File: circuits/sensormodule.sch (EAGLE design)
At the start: 9 parts, among them U1 ATMEGA328P_PDIP, Y1 16MHz

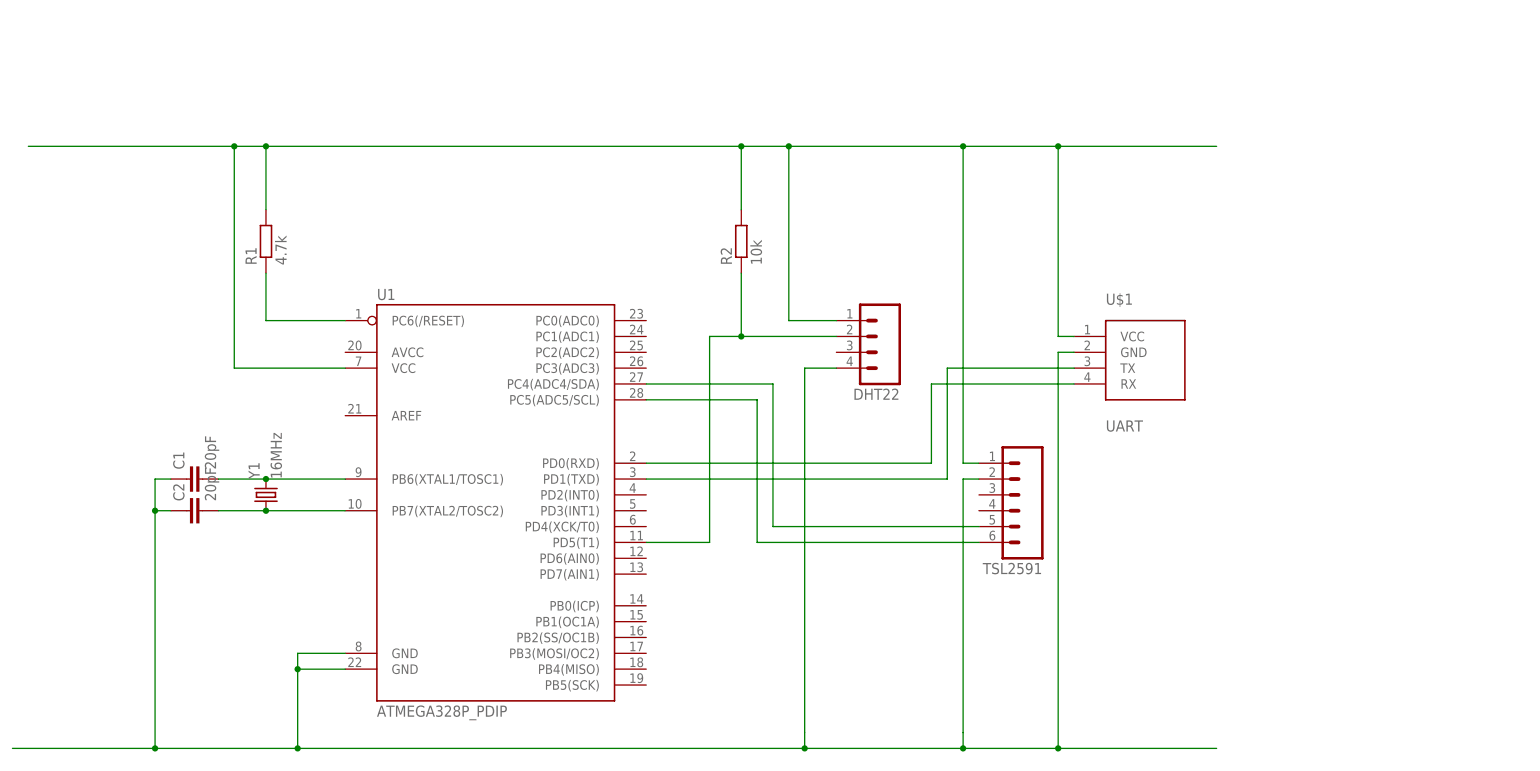
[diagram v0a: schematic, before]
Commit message: circuit update
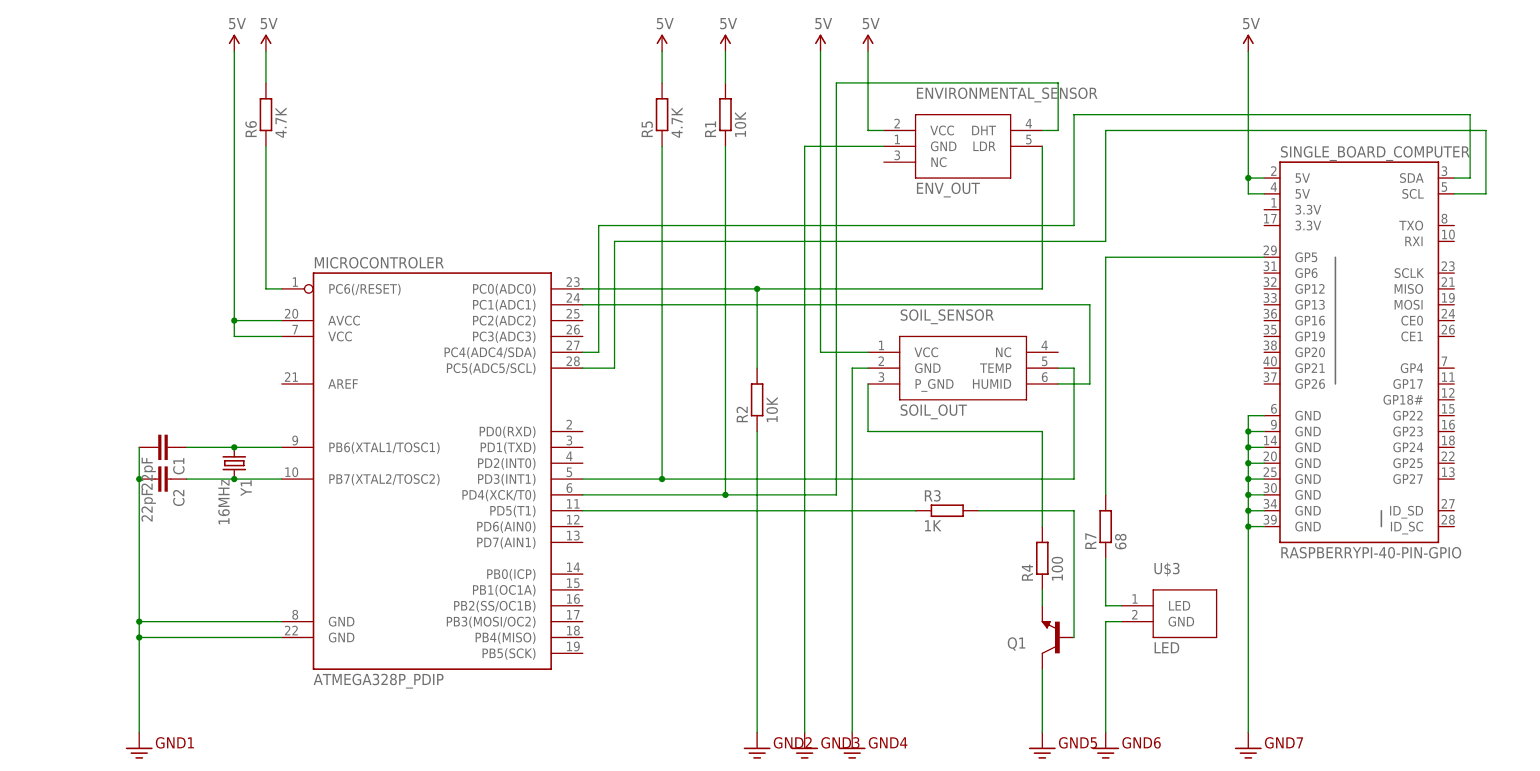
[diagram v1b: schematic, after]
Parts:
- removed DHT22: (no value), 001_SparkFun-Connectors:M04LOCK_LONGPADS
- removed TSL2591: (no value), 001_SparkFun-Connectors:M06LOCK_LONGPADS
- removed U$1: UART, 000_CropQuant:UART
- removed U1: ATMEGA328P_PDIP, 001_SparkFun-DigitalIC:ATMEGA328P_PDIP
- added ENVIRONMENTAL_SENSOR: ENV_OUT, 000_CropQuant:ENV_OUT
- added MICROCONTROLER: ATMEGA328P_PDIP, SparkFun-DigitalIC:ATMEGA328P_PDIP
- added Q1: (no value), SparkFun-DiscreteSemi:TRANSISTOR_NPNP2N2222A
- added R3: 1K, resistor:R-EU_0204/7
- added R4: 100, resistor:R-EU_0204/7
- added R5, R6: 4.7K, resistor:R-EU_0204/7
- added R7: 68, resistor:R-EU_0204/7
- added SINGLE_BOARD_COMPUTER: RASPBERRYPI-40-PIN-GPIO, 001_SparkFun-Boards:RASPBERRYPI-40-PIN-GPIO
- added SOIL_SENSOR: SOIL_OUT, 000_CropQuant:SOIL_OUT
- added U$3: LED, 000_CropQuant:LED
- C1, C2: value 20pF -> 22pF; device 001_SparkFun-Capacitors:CAPPTH -> SparkFun-Capacitors:CAPPTH
- R1: value 4.7k -> 10K
- R2: value 10k -> 10K
- Y1: device 001_SparkFun-FreqCtrl:CRYSTALHC49US -> SparkFun-FreqCtrl:CRYSTALHC49US
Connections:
- new net 3.3V: C1.2, C2.2, ENVIRONMENTAL_SENSOR.GND, MICROCONTROLER.GND@1, MICROCONTROLER.GND@2, Q1.C, R2.1, SINGLE_BOARD_COMPUTER.GND@14, SINGLE_BOARD_COMPUTER.GND@20, SINGLE_BOARD_COMPUTER.GND@25, SINGLE_BOARD_COMPUTER.GND@30, SINGLE_BOARD_COMPUTER.GND@34, SINGLE_BOARD_COMPUTER.GND@39, SINGLE_BOARD_COMPUTER.GND@6, SINGLE_BOARD_COMPUTER.GND@9, SOIL_SENSOR.GND, U$3.GND
- new net 5V: ENVIRONMENTAL_SENSOR.VCC, MICROCONTROLER.AVCC, MICROCONTROLER.VCC, R1.2, R5.2, R6.2, SINGLE_BOARD_COMPUTER.5V@2, SINGLE_BOARD_COMPUTER.5V@4, SOIL_SENSOR.VCC
- new net N$11: MICROCONTROLER.PC1(ADC1), SOIL_SENSOR.HUMID
- new net N$12: MICROCONTROLER.PC5(ADC5/SCL), SINGLE_BOARD_COMPUTER.SCL
- new net N$15: MICROCONTROLER.PC6(/RESET), R6.1
- new net N$16: R7.1, U$3.LED
- new net N$17: R7.2, SINGLE_BOARD_COMPUTER.GP5
- net N$1: now also C1.1, MICROCONTROLER.PB6(XTAL1/TOSC1), Y1.1; no longer R1.1, U1.PC6(/RESET)
- net N$10: now also R4.2, SOIL_SENSOR.P_GND; no longer U$1.RX, U1.PD0(RXD)
- net N$2: now also C2.1, MICROCONTROLER.PB7(XTAL2/TOSC2); no longer C1.2, U1.PB6(XTAL1/TOSC1)
- net N$3: now also Q1.E, R4.1; no longer C2.2, U1.PB7(XTAL2/TOSC2), Y1.1
- net N$4: now also ENVIRONMENTAL_SENSOR.LDR, MICROCONTROLER.PC0(ADC0); no longer DHT22.1, R1.2, TSL2591.1, U$1.VCC, U1.VCC
- net N$5: now also MICROCONTROLER.PC4(ADC4/SDA), SINGLE_BOARD_COMPUTER.SDA; no longer DHT22.2, R2.1, U1.PD5(T1)
- net N$6: now also MICROCONTROLER.PD3(INT1), R5.1, SOIL_SENSOR.TEMP; no longer C1.1, C2.1, DHT22.4, TSL2591.2, U$1.GND, U1.GND@1, U1.GND@2
- net N$7: now also ENVIRONMENTAL_SENSOR.DHT, MICROCONTROLER.PD4(XCK/T0), R1.1; no longer TSL2591.5, U1.PC4(ADC4/SDA)
- net N$8: now also MICROCONTROLER.PD5(T1), R3.1; no longer TSL2591.6, U1.PC5(ADC5/SCL)
- net N$9: now also Q1.B, R3.2; no longer U$1.TX, U1.PD1(TXD)
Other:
- note added: "CropQuant All-in-one HAT - BAYER 09.2017"
- moved on the sheet: C1, C2, R1, R2, Y1
